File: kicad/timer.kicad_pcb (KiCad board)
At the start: 2 copper layers, 10 parts, among them IC1 ATMEGA328P-A, U1 TOUCH_PAD_13, U2 MTCH6102_SSOP

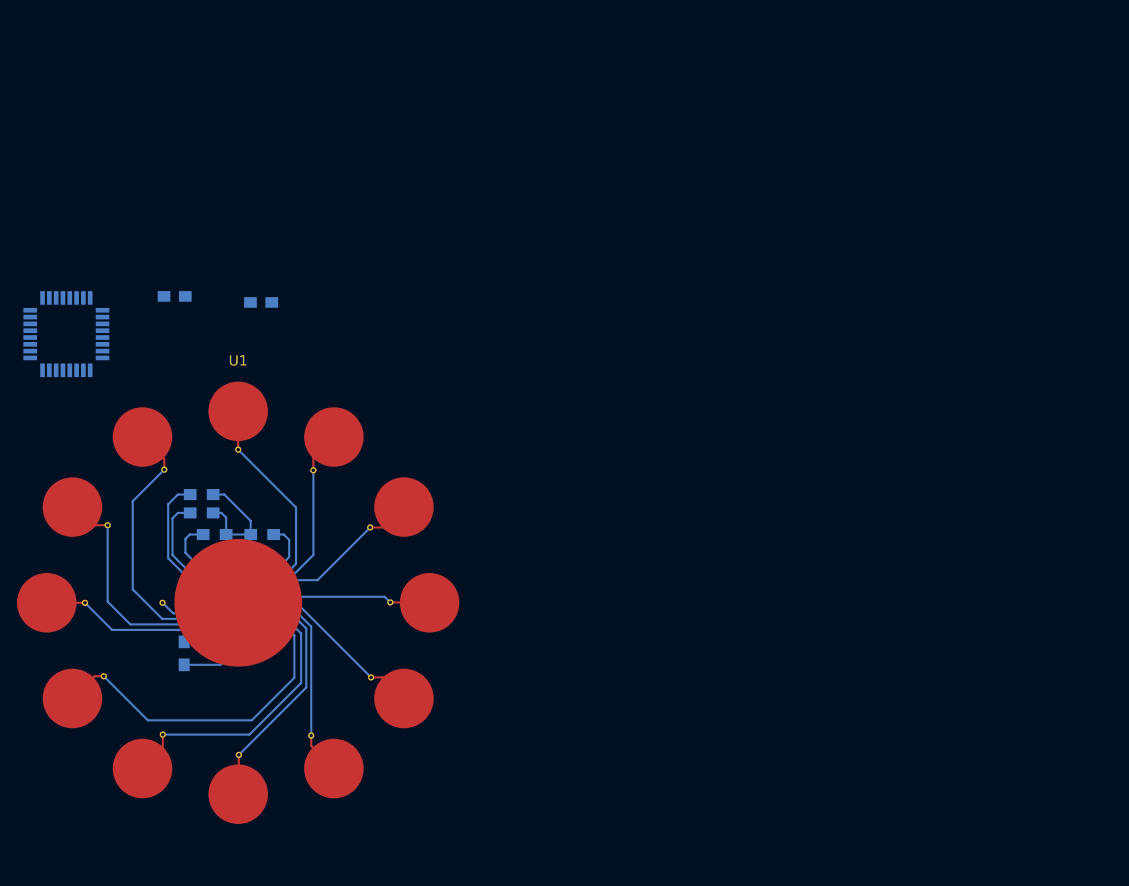
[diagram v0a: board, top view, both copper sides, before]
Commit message: Sqeeze it in
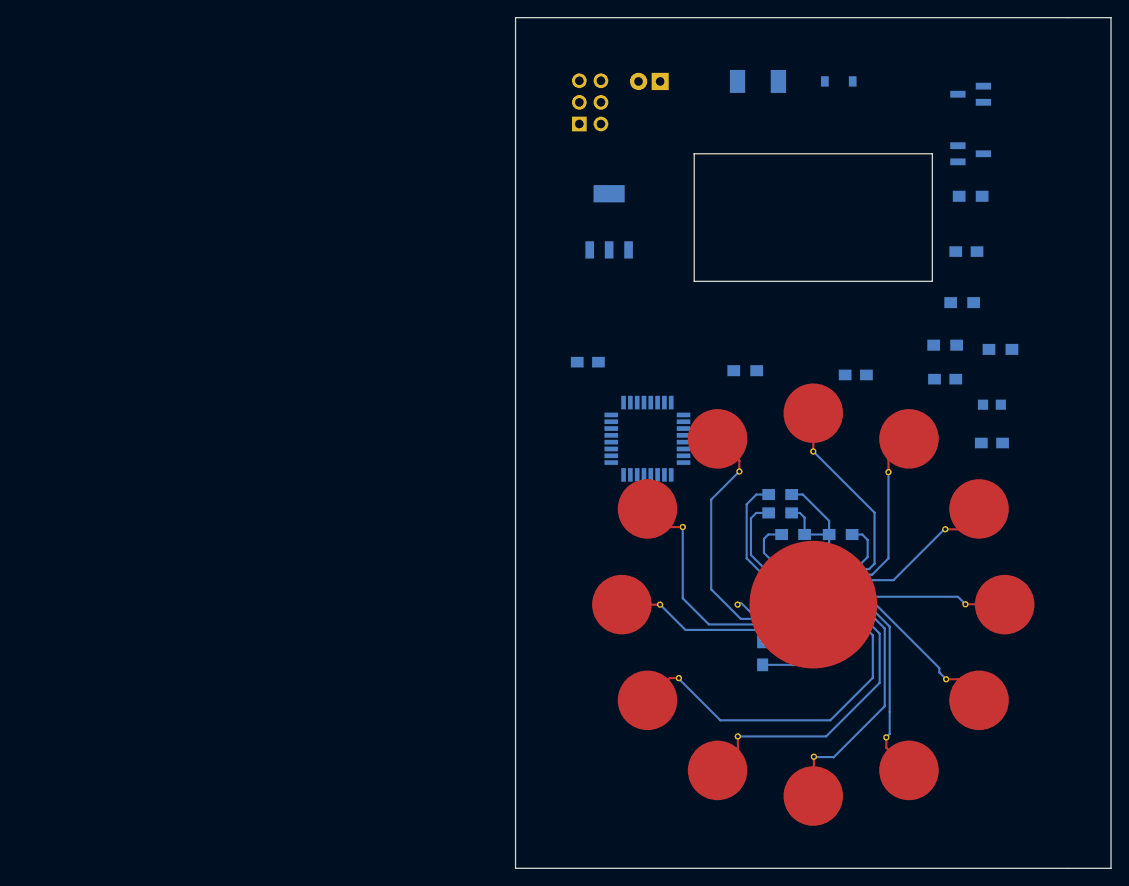
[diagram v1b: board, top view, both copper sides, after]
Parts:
- added C3: 1uF, Capacitors_SMD:C_0805_HandSoldering, B.Cu at (168.0, 62.5)
- added C4: 1uF, Capacitors_SMD:C_0805_HandSoldering, B.Cu at (155.0, 77.0)
- added C5: 0.1uF, Capacitors_SMD:C_0805_HandSoldering, B.Cu at (171.0, 85.0)
- added D1: D_Schottky, Diodes_SMD:SOD-123, B.Cu at (153.0, 42.5)
- added D2: Led, LEDs:LED_0805, B.Cu at (171.0, 80.5)
- added P1: BATTERY, Pin_Headers:Pin_Header_Straight_1x02, B.Cu at (132.0, 42.5)
- added P2: ICSP, Pin_Headers:Pin_Header_Straight_2x03, B.Cu at (122.5, 47.5)
- added Q1: NMOS, TO_SOT_Packages_SMD:SOT-23_Handsoldering, B.Cu at (168.5, 44.0)
- added Q2: PMOS, TO_SOT_Packages_SMD:SOT-23_Handsoldering, B.Cu at (168.5, 51.0)
- added R10: 100k, Resistors_SMD:R_0805_HandSoldering, B.Cu at (167.5, 68.5)
- added R6: 220, Resistors_SMD:R_0805_HandSoldering, B.Cu at (142.0, 76.5)
- added R7: 10K, Resistors_SMD:R_0805_HandSoldering, B.Cu at (165.5, 73.5)
- added R8: 100K, Resistors_SMD:R_0805_HandSoldering, B.Cu at (168.5, 56.0)
- added R9: 820, Resistors_SMD:R_0805_HandSoldering, B.Cu at (172.0, 74.0)
- added SW1: SPST, SMD_Packages:SMD-2010_Pol, B.Cu at (143.5, 42.5)
- added U3: MCP1755ST-3302E/DB, TO_SOT_Packages_SMD:SOT-223, B.Cu at (126.0, 59.0)
- moved C1 91.1 mm to (165.5, 77.5)
- moved IC1 69.4 mm to (130.5, 84.5)
- moved R3 68.0 mm to (153.2, 95.8)
- moved U2 68.0 mm to (150.6, 103.4)
- moved R1 68.0 mm to (144.0, 109.7)
- moved R2 68.0 mm to (147.6, 95.8)
- moved R4 68.0 mm to (146.1, 91.1)
- moved R5 68.0 mm to (146.1, 93.2)
- moved U1 67.6 mm to (150.0, 104.0)
- moved C2 39.0 mm to (123.5, 75.5)
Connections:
- C1 pad 1: VCC -> /3V3
- C2 pad 1: VCC -> /3V3
- IC1 pad 13: Net-(IC1-Pad13) -> /NBASE_ON
- IC1 pad 15: Net-(IC1-Pad15) -> /MOSI
- IC1 pad 16: Net-(IC1-Pad16) -> /MISO
- IC1 pad 17: Net-(IC1-Pad17) -> /SCK
- IC1 pad 21: Net-(IC1-Pad21) -> GND
- IC1 pad 29: Net-(IC1-Pad29) -> /RESET
- IC1 pad 3: Net-(IC1-Pad3) -> GND
- IC1 pad 4: Net-(IC1-Pad4) -> /3V3
- IC1 pad 5: Net-(IC1-Pad5) -> GND
- IC1 pad 6: Net-(IC1-Pad6) -> /3V3
- R1 pad 1: VCC -> /3V3
- R2 pad 1: VCC -> /3V3
- R3 pad 1: VCC -> /3V3
- R4 pad 1: VCC -> Net-(R4-Pad1)
- R5 pad 1: VCC -> /3V3
- U2 pad 20: VCC -> /3V3
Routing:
- net VCC: track 38.4 -> 0.00 mm
- net /3V3: track 0.00 -> 37.1 mm
- net /RX4: track 20.4 -> 23.9 mm
- net /RX1: track 20.9 -> 24.0 mm
- net /RX2: track 19.2 -> 22.2 mm
- net /RX6: track 27.7 -> 29.7 mm
- net Net-(R4-Pad1): track 0.00 -> 1.32 mm
- net /RX7: track 33.9 -> 34.6 mm
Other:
- board outline added: 70 x 100 mm
